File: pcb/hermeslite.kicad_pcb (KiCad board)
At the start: 4 copper layers, 49.9 x 49.9 mm, 71 parts, among them CN1 MEC6-140_CONNECTOR_BEMICRO, CN2 PCIE, CN3 SATA22, J1 0, J2 0, J3 0, J4 0, J5 0, P0 CONN_1, P12 CONN_1, P3 CONN_1, P5 CONN_1, U1 AD9866BCPZ, U2 EEPROM, X1 61.440

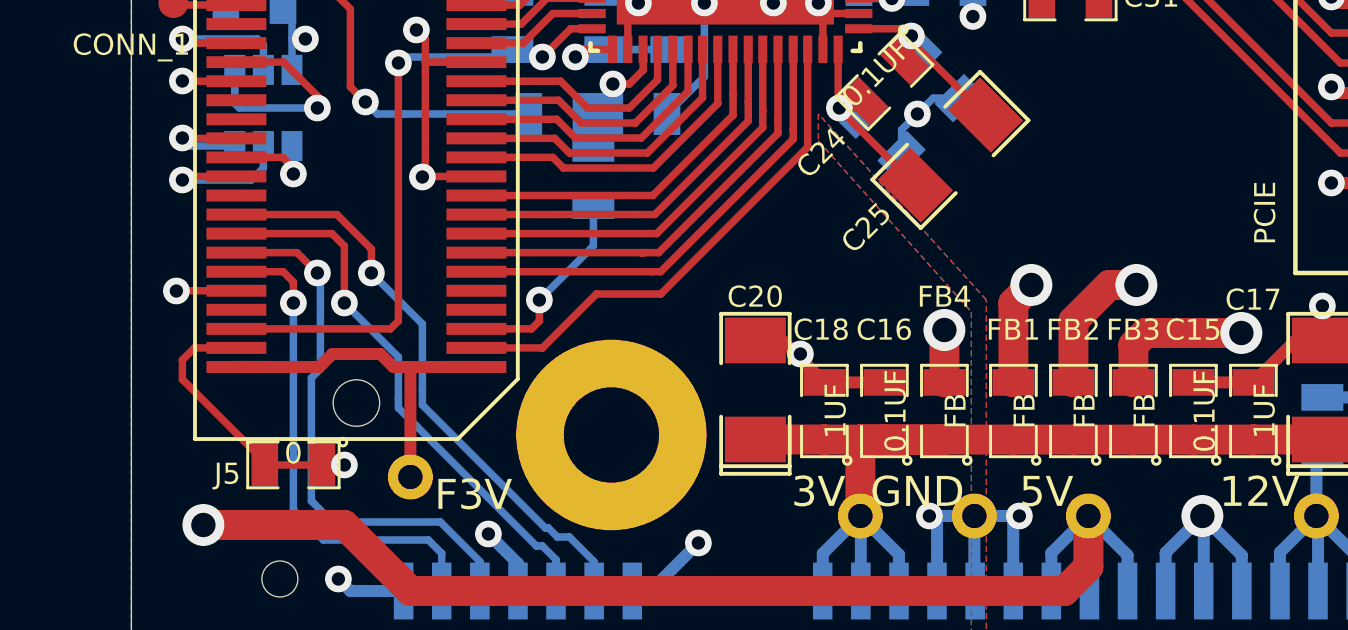
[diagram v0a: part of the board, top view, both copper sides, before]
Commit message: iTead Studio submission
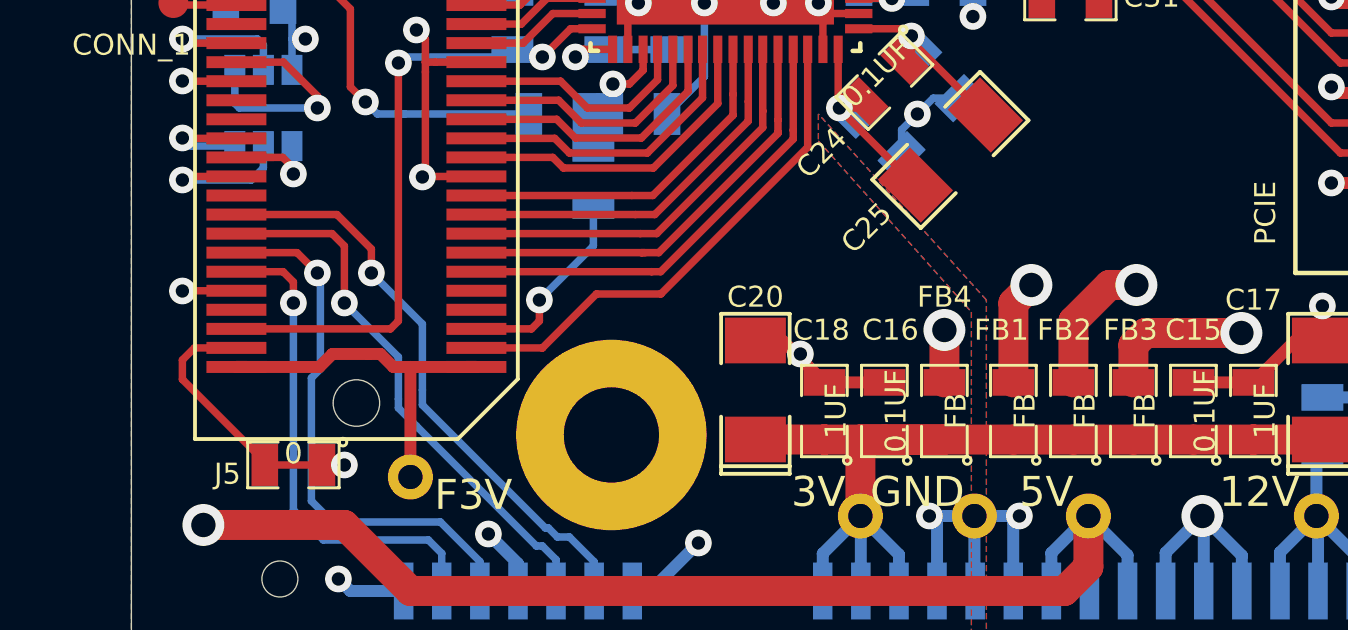
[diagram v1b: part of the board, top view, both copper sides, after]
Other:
- net class Default: clearance 0.205 -> 0
- rule trace_clearance: 0.205 -> 0
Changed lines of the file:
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@@
   (title_block
     (title Hermes-Lite)
-    (date "07 Oct 2014")
+    (date "08 Oct 2014")
     (rev 1,2)
     (company SofterHardware)
@@
   (layers
     (0 F.Cu signal)
-    (1 Inner2.Cu signal hide)
-    (2 Inner1.Cu signal hide)
-    (31 B.Cu signal hide)
+    (1 Inner2.Cu signal)
+    (2 Inner1.Cu signal)
+    (31 B.Cu signal)
     (32 B.Adhes user)
     (33 F.Adhes user)
@@
     (35 F.Paste user)
     (36 B.SilkS user)
-    (37 F.SilkS user hide)
+    (37 F.SilkS user)
     (38 B.Mask user)
     (39 F.Mask user)
@@
     (user_trace_width 0.4)
     (user_trace_width 1)
-    (trace_clearance 0.205)
+    (trace_clearance 0)
     (zone_clearance 0.45)
     (zone_45_only no)
@@
     (pad_drill 0.813)
     (pad_to_mask_clearance 0)
-    (aux_axis_origin 100.7 83.45)
+    (aux_axis_origin 100.7 83.2)
     (visible_elements FFFEFF7F)
     (pcbplotparams
-      (layerselection 0x01030_80000007)
+      (layerselection 0x010f0_80000007)
       (usegerberextensions true)
-      (excludeedgelayer true)
+      (excludeedgelayer false)
       (linewidth 0.150000)
       (plotframeref false)
@@
   (net 94 "Net-(R1-Pad2)")
   (net_class Default "This is the default net class."
-    (clearance 0.205)
+    (clearance 0)
     (trace_width 0.25)
     (via_dia 0.889)
@@
     (pad B18 smd rect (at -7.5 3.5 270) (size 0.7 3) (layers F.Cu F.Paste F.Mask)
       (net 81 /EXP_SCLK))
-    (pad A1 smd rect (at 11.5 3.5 270) (size 0.7 3) (layers B.Cu F.Paste F.Mask)
-      (net 5 GND))
-    (pad A2 smd rect (at 10.5 3.5 270) (size 0.7 3) (layers B.Cu F.Paste F.Mask)
-      (net 5 GND))
-    (pad A3 smd rect (at 9.5 3.5 270) (size 0.7 3) (layers B.Cu F.Paste F.Mask)
-      (net 5 GND))
-    (pad A4 smd rect (at 8.5 3.5 270) (size 0.7 3) (layers B.Cu F.Paste F.Mask)
-      (net 5 GND))
-    (pad A5 smd rect (at 7.5 3.5 270) (size 0.7 3) (layers B.Cu F.Paste F.Mask)
-      (net 5 GND))
-    (pad A6 smd rect (at 6.5 3.5 270) (size 0.7 3) (layers B.Cu F.Paste F.Mask)
-      (net 5 GND))
-    (pad A7 smd rect (at 5.5 3.5 270) (size 0.7 3) (layers B.Cu F.Paste F.Mask)
-      (net 5 GND))
-    (pad A8 smd rect (at 4.5 3.5 270) (size 0.7 3) (layers B.Cu F.Paste F.Mask)
-      (net 5 GND))
-    (pad A9 smd rect (at 3.5 3.5 270) (size 0.7 3) (layers B.Cu F.Paste F.Mask)
-      (net 5 GND))
-    (pad A10 smd rect (at 2.5 3.5 270) (size 0.7 3) (layers B.Cu F.Paste F.Mask)
-      (net 5 GND))
-    (pad A11 smd rect (at 1.5 3.5 270) (size 0.7 3) (layers B.Cu F.Paste F.Mask)
+    (pad A1 smd rect (at 11.5 3.5 270) (size 0.7 3) (layers B.Cu B.Paste B.Mask)
+      (net 5 GND))
+    (pad A2 smd rect (at 10.5 3.5 270) (size 0.7 3) (layers B.Cu B.Paste B.Mask)
+      (net 5 GND))
+    (pad A3 smd rect (at 9.5 3.5 270) (size 0.7 3) (layers B.Cu B.Paste B.Mask)
+      (net 5 GND))
+    (pad A4 smd rect (at 8.5 3.5 270) (size 0.7 3) (layers B.Cu B.Paste B.Mask)
+      (net 5 GND))
+    (pad A5 smd rect (at 7.5 3.5 270) (size 0.7 3) (layers B.Cu B.Paste B.Mask)
+      (net 5 GND))
+    (pad A6 smd rect (at 6.5 3.5 270) (size 0.7 3) (layers B.Cu B.Paste B.Mask)
+      (net 5 GND))
+    (pad A7 smd rect (at 5.5 3.5 270) (size 0.7 3) (layers B.Cu B.Paste B.Mask)
+      (net 5 GND))
+    (pad A8 smd rect (at 4.5 3.5 270) (size 0.7 3) (layers B.Cu B.Paste B.Mask)
+      (net 5 GND))
+    (pad A9 smd rect (at 3.5 3.5 270) (size 0.7 3) (layers B.Cu B.Paste B.Mask)
+      (net 5 GND))
+    (pad A10 smd rect (at 2.5 3.5 270) (size 0.7 3) (layers B.Cu B.Paste B.Mask)
+      (net 5 GND))
+    (pad A11 smd rect (at 1.5 3.5 270) (size 0.7 3) (layers B.Cu B.Paste B.Mask)
       (net 91 EXP12V))
-    (pad A12 smd rect (at -1.5 3.5 270) (size 0.7 3) (layers B.Cu F.Paste F.Mask)
+    (pad A12 smd rect (at -1.5 3.5 270) (size 0.7 3) (layers B.Cu B.Paste B.Mask)
       (net 91 EXP12V))
-    (pad A13 smd rect (at -2.5 3.5 270) (size 0.7 3) (layers B.Cu F.Paste F.Mask)
+    (pad A13 smd rect (at -2.5 3.5 270) (size 0.7 3) (layers B.Cu B.Paste B.Mask)
       (net 92 EXP5V))
-    (pad A14 smd rect (at -3.5 3.5 270) (size 0.7 3) (layers B.Cu F.Paste F.Mask)
+    (pad A14 smd rect (at -3.5 3.5 270) (size 0.7 3) (layers B.Cu B.Paste B.Mask)
       (net 92 EXP5V))
-    (pad A15 smd rect (at -4.5 3.5 270) (size 0.7 3) (layers B.Cu F.Paste F.Mask)
+    (pad A15 smd rect (at -4.5 3.5 270) (size 0.7 3) (layers B.Cu B.Paste B.Mask)
       (net 93 EXP3V))
-    (pad A16 smd rect (at -5.5 3.5 270) (size 0.7 3) (layers B.Cu F.Paste F.Mask)
+    (pad A16 smd rect (at -5.5 3.5 270) (size 0.7 3) (layers B.Cu B.Paste B.Mask)
       (net 93 EXP3V))
-    (pad A17 smd rect (at -6.5 3.5 270) (size 0.7 3) (layers B.Cu F.Paste F.Mask)
-      (net 5 GND))
-    (pad A18 smd rect (at -7.5 3.5 270) (size 0.7 3) (layers B.Cu F.Paste F.Mask)
+    (pad A17 smd rect (at -6.5 3.5 270) (size 0.7 3) (layers B.Cu B.Paste B.Mask)
+      (net 5 GND))
+    (pad A18 smd rect (at -7.5 3.5 270) (size 0.7 3) (layers B.Cu B.Paste B.Mask)
       (net 5 GND))
   )
@@
     (at 130.1 122 90)
     (attr smd)
-    (fp_text reference FB1 (at 2.7 0 180) (layer F.SilkS)
+    (fp_text reference FB1 (at 2.7 -0.4 180) (layer F.SilkS)
       (effects (font (size 0.7 0.7) (thickness 0.1)))
     )
@@
     (at 132.1 122 90)
     (attr smd)
-    (fp_text reference FB2 (at 2.7 0 180) (layer F.SilkS)
+    (fp_text reference FB2 (at 2.7 -0.3 180) (layer F.SilkS)
       (effects (font (size 0.7 0.7) (thickness 0.1)))
     )
@@
     (at 134.1 122 90)
     (attr smd)
-    (fp_text reference FB3 (at 2.7 0 180) (layer F.SilkS)
+    (fp_text reference FB3 (at 2.7 -0.1 180) (layer F.SilkS)
       (effects (font (size 0.7 0.7) (thickness 0.1)))
     )
@@
     (at 125.8 122 90)
     (attr smd)
-    (fp_text reference C16 (at 2.7 0 180) (layer F.SilkS)
+    (fp_text reference C16 (at 2.7 0.2 180) (layer F.SilkS)
       (effects (font (size 0.7 0.7) (thickness 0.1)))
     )
@@
   (via (at 102.375 104.025) (size 0.889) (layers F.Cu B.Cu) (net 5))
   (segment (start 104.2 104.0225) (end 102.3775 104.0225) (width 0.25) (layer F.Cu) (net 5))
-  (segment (start 102.2075 117.9925) (end 102.2 118) (width 0.25) (layer F.Cu) (net 5))
-  (via (at 102.2 118) (size 0.889) (layers F.Cu B.Cu) (net 5))
-  (segment (start 104.2 117.9925) (end 102.2075 117.9925) (width 0.25) (layer F.Cu) (net 5))
   (segment (start 105.1 113.9) (end 104.7 114.3) (width 0.25) (layer B.Cu) (net 5))
   (segment (start 104.7 114.3) (end 102.4 114.3) (width 0.25) (layer B.Cu) (net 5))
@@
   (via (at 136.4 125.5) (size 1.397) (drill 0.813) (layers F.Cu B.Cu) (net 5))
   (segment (start 137.715 128) (end 137.715 126.815) (width 0.4) (layer B.Cu) (net 5))
+  (segment (start 102.4075 117.9925) (end 102.4 118) (width 0.25) (layer F.Cu) (net 5))
+  (via (at 102.4 118) (size 0.889) (layers F.Cu B.Cu) (net 5))
+  (segment (start 104.2 117.9925) (end 102.4075 117.9925) (width 0.25) (layer F.Cu) (net 5))
   (segment (start 126.7 110.1) (end 126.473519 110.326481) (width 0.25) (layer F.Cu) (net 6))
   (segment (start 126.7 109.5) (end 126.7 110.1) (width 0.25) (layer F.Cu) (net 6))
